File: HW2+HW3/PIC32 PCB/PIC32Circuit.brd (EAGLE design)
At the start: 50 x 50 mm, 22 parts, among them J1 USB-MB-H

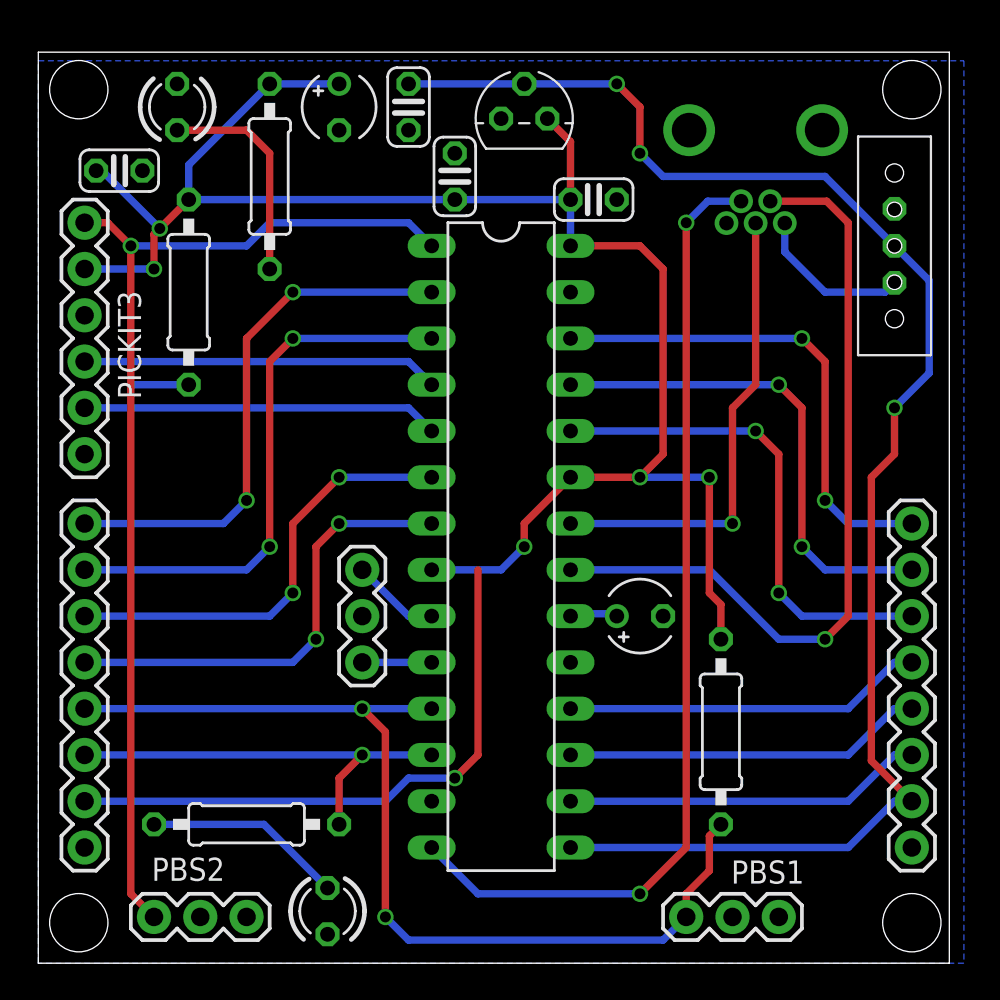
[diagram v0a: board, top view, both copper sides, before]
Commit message: Ready to be checked before order
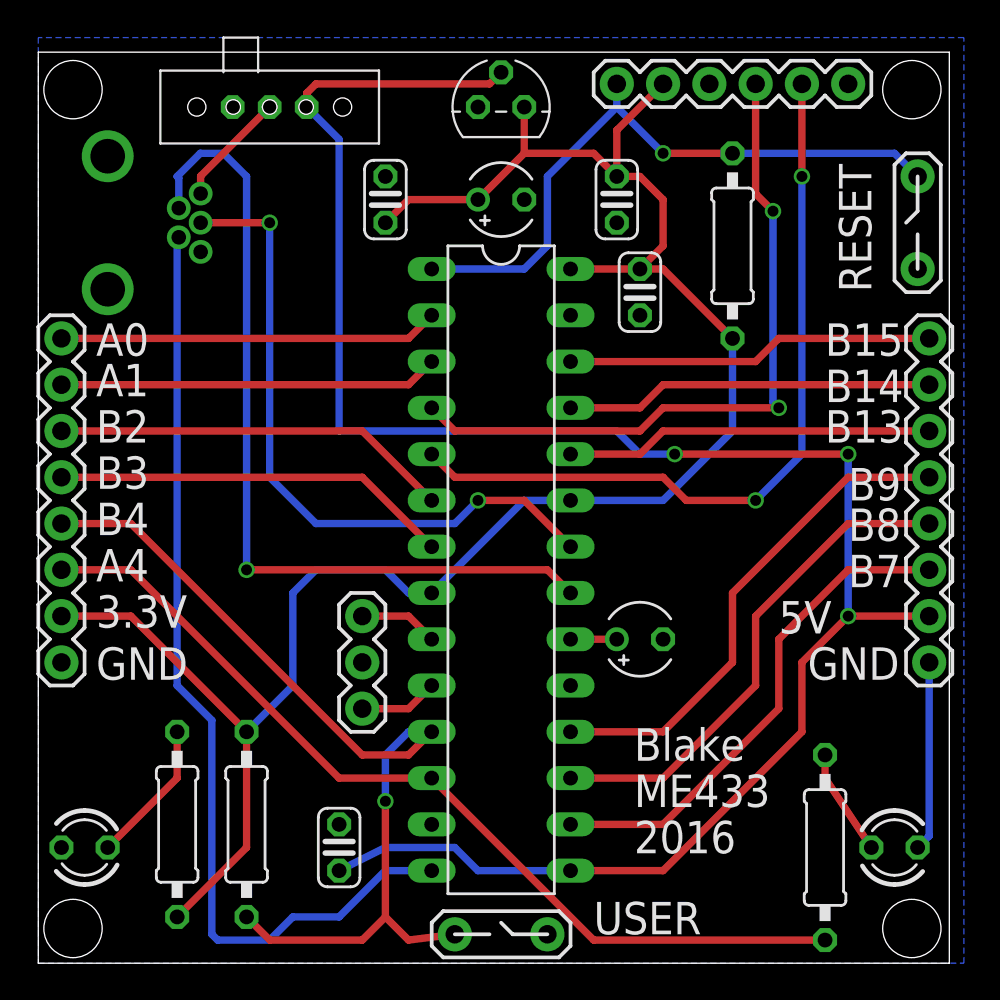
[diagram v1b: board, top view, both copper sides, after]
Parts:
- removed PBS1, PBS2: (no value), PIC32:1X03
- added RESET, USER: PUSHBUTTON, PIC32:PUSHBUTTON
- C1, C2: value 1uF -> 0.1uF
- C3: value .1uF -> 0.1uF
- moved LED1 41.0 mm to (2.54, 6.35), turned to 180 degrees
- moved C1 40.8 mm to (16.5, 6.35), turned to 90 degrees
- moved R4 35.9 mm to (7.62, 7.62), turned to 90 degrees
- moved J1 35.9 mm to (3.81, 40.6), turned to 0 degrees
- moved U$2 35.1 mm to (12.7, 47.0), turned to 90 degrees
- moved R5 31.8 mm to (43.2, 6.35), turned to 90 degrees
- moved LED3 31.3 mm to (47.0, 6.35), turned to 0 degrees
- moved PICKIT3 30.2 mm to (31.8, 48.3), turned to 0 degrees
- moved R1 30.0 mm to (38.1, 39.4), turned to 90 degrees
- moved R2 26.5 mm to (11.4, 7.62)
- moved C4 14.7 mm to (19.1, 41.9), turned to 90 degrees
- moved C3 12.0 mm to (33.0, 36.8), turned to 270 degrees
- moved C5 10.2 mm to (25.4, 41.9), turned to 0 degrees
- moved J5 10.2 mm to (1.27, 34.3)
- moved J4 10.2 mm to (48.9, 34.3)
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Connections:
- net 5V: now also U$2.P$3; no longer U$2.P$2
- net B4: now also USER.1; no longer PBS1.1
- net GND: now also RESET.1, USER.3; no longer PBS1.3, PBS2.1
- net MCLR: now also RESET.3; no longer PBS2.3
- net N$4: now also U$2.P$2; no longer U$2.P$3
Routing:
- net A4: track 23.4 -> 50.3 mm, vias 1 -> 0
- net MCLR: track 61.2 -> 35.4 mm
- net 5V: track 85.1 -> 109.0 mm
- net PGC: track 19.6 -> 42.7 mm, vias 0 -> 2
- net 3V3: track 131.3 -> 108.5 mm, vias 6 -> 0
- net PGD: track 19.6 -> 38.4 mm, vias 0 -> 2
- net D+: track 25.9 -> 36.9 mm, vias 1 -> 2
- net GND: track 0.00 -> 10.4 mm
- net A1: track 30.3 -> 20.8 mm, vias 2 -> 0
- net A0: track 29.5 -> 20.8 mm, vias 2 -> 0
- net B9: track 19.8 -> 27.7 mm
- net B8: track 19.8 -> 27.7 mm
- net B7: track 19.8 -> 27.7 mm
- net B15: track 27.4 -> 20.2 mm, vias 2 -> 0
- net B14: track 27.4 -> 20.2 mm, vias 2 -> 0
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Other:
- board text added: "2016"
- board text added: "3.3V"
- board text added: "5V"
- board text added: "A0"
- board text added: "A1"
- board text added: "A4"
- board text added: "B13"
- board text added: "B14"
- board text added: "B15"
- board text added: "B2"
- board text added: "B3"
- board text added: "B4"
- board text added: "B7"
- board text added: "B8"
- board text added: "B9"
- board text added: "Blake"
- board text added: "GND"
- board text added: "ME433"
- board text added: "RESET"
- board text added: "USER"
